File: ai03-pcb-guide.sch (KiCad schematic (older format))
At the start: 16 parts

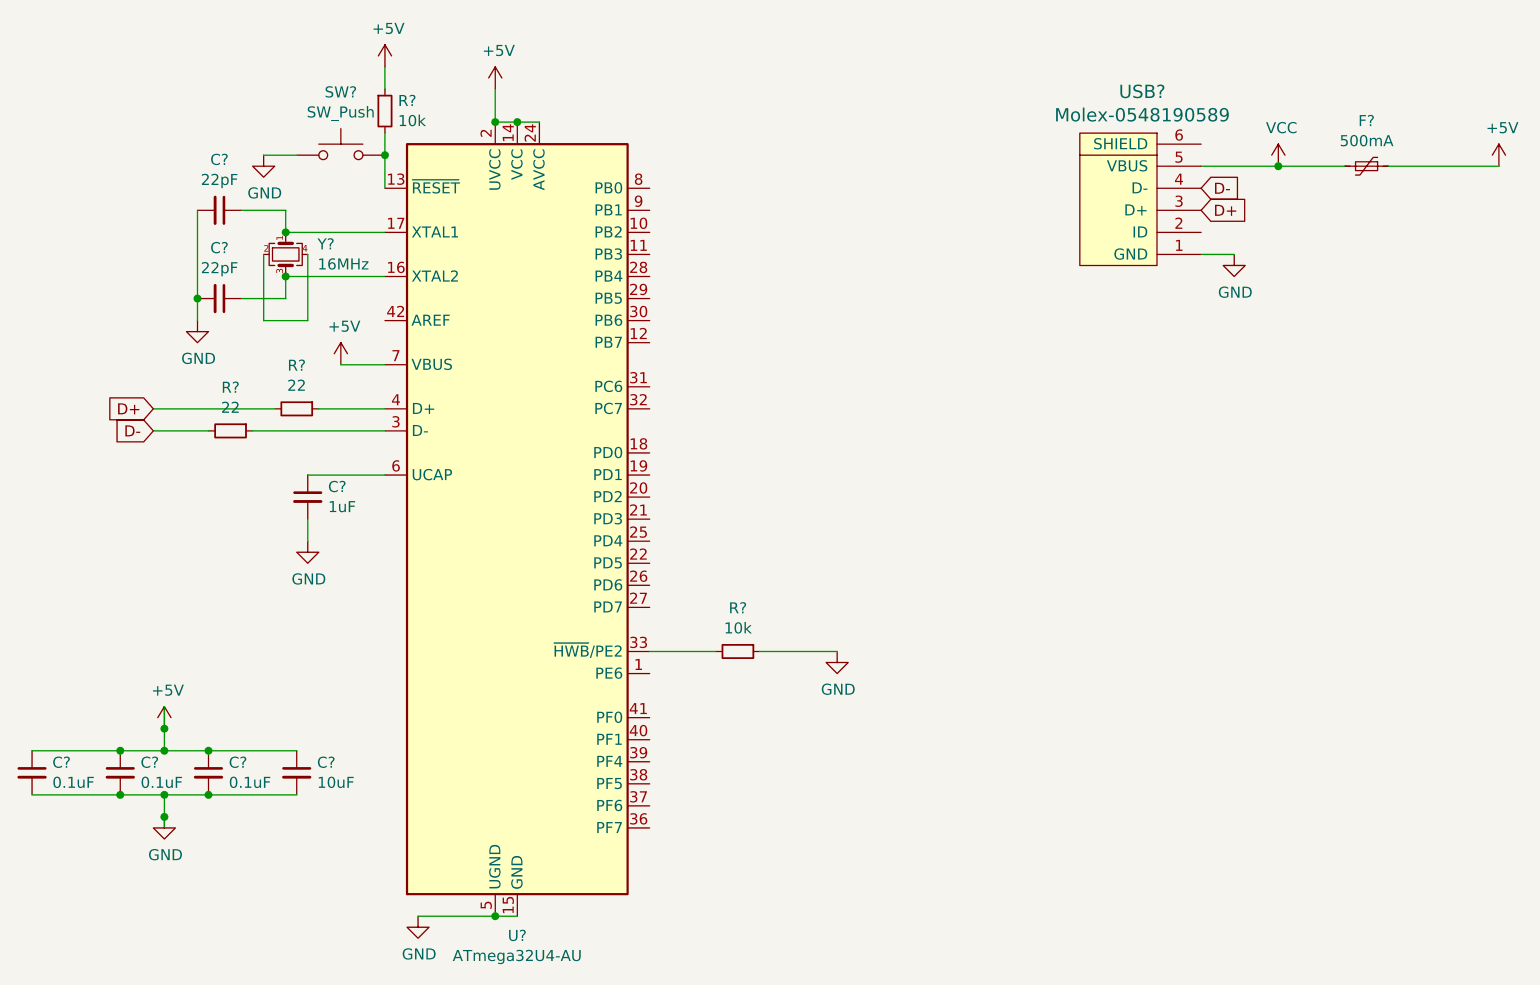
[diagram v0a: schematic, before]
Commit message: Switch schematic
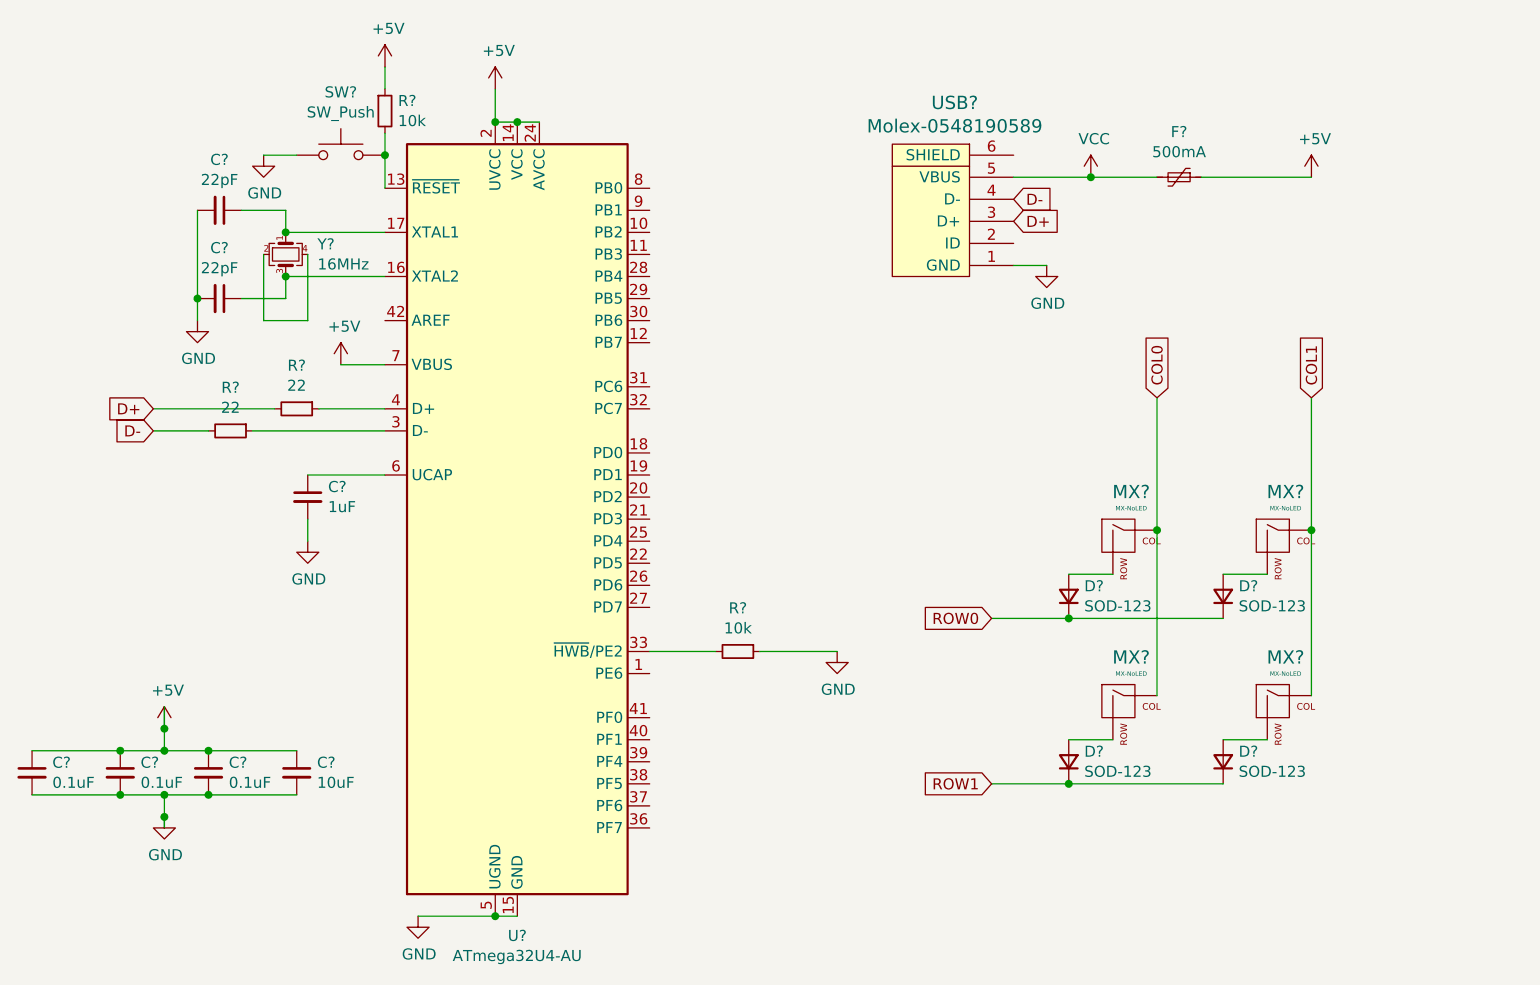
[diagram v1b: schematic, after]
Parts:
- added D? (x4): SOD-123, symbol Device:D_Small
- added MX? (x4): MX-NoLED, symbol MX_Alps_Hybrid:MX-NoLED
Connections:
- net labels added: COL0, COL1, ROW0, ROW1
- wire segments 45 -> 57
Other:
- moved on the sheet: F?, USB?
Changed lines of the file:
@@
 L random-keyboard-parts:Molex-0548190589 USB?
 U 1 1 6038615F
-P 6300 2400
-F 0 "USB?" V 6837 2367 60  0000 C CNN
-F 1 "Molex-0548190589" V 6731 2367 60  0000 C CNN
-F 2 "" H 6300 2400 60  0001 C CNN
-F 3 "" H 6300 2400 60  0001 C CNN
-	1    6300 2400
+P 5450 2450
+F 0 "USB?" V 5987 2417 60  0000 C CNN
+F 1 "Molex-0548190589" V 5881 2417 60  0000 C CNN
+F 2 "" H 5450 2450 60  0001 C CNN
+F 3 "" H 5450 2450 60  0001 C CNN
+	1    5450 2450
 	0    -1   -1   0
 $EndComp
@@
 L Device:Polyfuse_Small F?
 U 1 1 60388AFC
-P 7350 2200
-F 0 "F?" V 7145 2200 50  0000 C CNN
-F 1 "500mA" V 7236 2200 50  0000 C CNN
-F 2 "" H 7400 2000 50  0001 L CNN
-F 3 "~" H 7350 2200 50  0001 C CNN
-	1    7350 2200
+P 6500 2250
+F 0 "F?" V 6295 2250 50  0000 C CNN
+F 1 "500mA" V 6386 2250 50  0000 C CNN
+F 2 "" H 6550 2050 50  0001 L CNN
+F 3 "~" H 6500 2250 50  0001 C CNN
+	1    6500 2250
 	0    1    1    0
 $EndComp
 Wire Wire Line
-	6600 2200 6950 2200
+	5750 2250 6100 2250
 $Comp
 L power:VCC #PWR?
 U 1 1 6038C6B9
-P 6950 2200
-F 0 "#PWR?" H 6950 2050 50  0001 C CNN
-F 1 "VCC" H 6965 2373 50  0000 C CNN
-F 2 "" H 6950 2200 50  0001 C CNN
-F 3 "" H 6950 2200 50  0001 C CNN
-	1    6950 2200
+P 6100 2250
+F 0 "#PWR?" H 6100 2100 50  0001 C CNN
+F 1 "VCC" H 6115 2423 50  0000 C CNN
+F 2 "" H 6100 2250 50  0001 C CNN
+F 3 "" H 6100 2250 50  0001 C CNN
+	1    6100 2250
 	1    0    0    -1
 $EndComp
-Connection ~ 6950 2200
+Connection ~ 6100 2250
 Wire Wire Line
-	6950 2200 7250 2200
+	6100 2250 6400 2250
 Wire Wire Line
-	7450 2200 7950 2200
+	6600 2250 7100 2250
 $Comp
 L power:+5V #PWR?
 U 1 1 6038A873
-P 7950 2200
-F 0 "#PWR?" H 7950 2050 50  0001 C CNN
-F 1 "+5V" H 7965 2373 50  0000 C CNN
-F 2 "" H 7950 2200 50  0001 C CNN
-F 3 "" H 7950 2200 50  0001 C CNN
-	1    7950 2200
+P 7100 2250
+F 0 "#PWR?" H 7100 2100 50  0001 C CNN
+F 1 "+5V" H 7115 2423 50  0000 C CNN
+F 2 "" H 7100 2250 50  0001 C CNN
+F 3 "" H 7100 2250 50  0001 C CNN
+	1    7100 2250
 	1    0    0    -1
 $EndComp
-Text GLabel 6600 2400 2    50   Input ~ 0
+Text GLabel 5750 2450 2    50   Input ~ 0
 D+
-Text GLabel 6600 2300 2    50   Input ~ 0
+Text GLabel 5750 2350 2    50   Input ~ 0
 D-
 $Comp
 L power:GND #PWR?
 U 1 1 60394008
-P 6750 2600
-F 0 "#PWR?" H 6750 2350 50  0001 C CNN
-F 1 "GND" H 6755 2427 50  0000 C CNN
-F 2 "" H 6750 2600 50  0001 C CNN
-F 3 "" H 6750 2600 50  0001 C CNN
-	1    6750 2600
+P 5900 2650
+F 0 "#PWR?" H 5900 2400 50  0001 C CNN
+F 1 "GND" H 5905 2477 50  0000 C CNN
+F 2 "" H 5900 2650 50  0001 C CNN
+F 3 "" H 5900 2650 50  0001 C CNN
+	1    5900 2650
 	1    0    0    -1
 $EndComp
 Wire Wire Line
-	6600 2600 6750 2600
+	5750 2650 5900 2650
+$Comp
+L MX_Alps_Hybrid:MX-NoLED MX?
+U 1 1 60395692
+P 6250 3900
+F 0 "MX?" H 6283 4123 60  0000 C CNN
+F 1 "MX-NoLED" H 6283 4049 20  0000 C CNN
+F 2 "" H 5625 3875 60  0001 C CNN
+F 3 "" H 5625 3875 60  0001 C CNN
+	1    6250 3900
+	1    0    0    -1
+$EndComp
+$Comp
+L Device:D_Small D?
+U 1 1 6039B382
+P 6000 4150
+F 0 "D?" V 6046 4080 50  0000 R CNN
+F 1 "SOD-123" V 5955 4080 50  0000 R CNN
+F 2 "" V 6000 4150 50  0001 C CNN
+F 3 "~" V 6000 4150 50  0001 C CNN
+	1    6000 4150
+	0    -1   -1   0
+$EndComp
+Wire Wire Line
+	6200 4050 6000 4050
+$Comp
+L MX_Alps_Hybrid:MX-NoLED MX?
+U 1 1 603A0BDE
+P 6950 3900
+F 0 "MX?" H 6983 4123 60  0000 C CNN
+F 1 "MX-NoLED" H 6983 4049 20  0000 C CNN
+F 2 "" H 6325 3875 60  0001 C CNN
+F 3 "" H 6325 3875 60  0001 C CNN
+	1    6950 3900
+	1    0    0    -1
+$EndComp
+$Comp
+L Device:D_Small D?
+U 1 1 603A17C0
+P 6700 4150
+F 0 "D?" V 6746 4080 50  0000 R CNN
+F 1 "SOD-123" V 6655 4080 50  0000 R CNN
+F 2 "" V 6700 4150 50  0001 C CNN
+F 3 "~" V 6700 4150 50  0001 C CNN
+	1    6700 4150
+	0    -1   -1   0
+$EndComp
+Wire Wire Line
+	6900 4050 6700 4050
+$Comp
+L MX_Alps_Hybrid:MX-NoLED MX?
+U 1 1 603A2C50
+P 6250 4650
+F 0 "MX?" H 6283 4873 60  0000 C CNN
+F 1 "MX-NoLED" H 6283 4799 20  0000 C CNN
+F 2 "" H 5625 4625 60  0001 C CNN
+F 3 "" H 5625 4625 60  0001 C CNN
+	1    6250 4650
+	1    0    0    -1
+$EndComp
+$Comp
+L Device:D_Small D?
+U 1 1 603A36D6
+P 6000 4900
+F 0 "D?" V 6046 4830 50  0000 R CNN
+F 1 "SOD-123" V 5955 4830 50  0000 R CNN
+F 2 "" V 6000 4900 50  0001 C CNN
+F 3 "~" V 6000 4900 50  0001 C CNN
+	1    6000 4900
+	0    -1   -1   0
+$EndComp
+Wire Wire Line
+	6200 4800 6000 4800
+$Comp
+L MX_Alps_Hybrid:MX-NoLED MX?
+U 1 1 603A4940
+P 6950 4650
+F 0 "MX?" H 6983 4873 60  0000 C CNN
+F 1 "MX-NoLED" H 6983 4799 20  0000 C CNN
+F 2 "" H 6325 4625 60  0001 C CNN
+F 3 "" H 6325 4625 60  0001 C CNN
+	1    6950 4650
+	1    0    0    -1
+$EndComp
+$Comp
+L Device:D_Small D?
+U 1 1 603A51B7
+P 6700 4900
+F 0 "D?" V 6746 4830 50  0000 R CNN
+F 1 "SOD-123" V 6655 4830 50  0000 R CNN
+F 2 "" V 6700 4900 50  0001 C CNN
+F 3 "~" V 6700 4900 50  0001 C CNN
+	1    6700 4900
+	0    -1   -1   0
+$EndComp
+Wire Wire Line
+	6900 4800 6700 4800
+Wire Wire Line
+	7100 4600 7100 3850
+Connection ~ 7100 3850
+Wire Wire Line
+	7100 3850 7100 3250
+Wire Wire Line
+	6400 4600 6400 3850
+Connection ~ 6400 3850
+Wire Wire Line
+	6400 3850 6400 3250
+Wire Wire Line
+	6700 4250 6000 4250
+Connection ~ 6000 4250
+Wire Wire Line
+	6000 4250 5650 4250
+Wire Wire Line
+	6700 5000 6000 5000
+Connection ~ 6000 5000
+Wire Wire Line
+	6000 5000 5650 5000
+Text GLabel 6400 3250 1    50   Input ~ 0
+COL0
+Text GLabel 7100 3250 1    50   Input ~ 0
+COL1
+Text GLabel 5650 4250 0    50   Input ~ 0
+ROW0
+Text GLabel 5650 5000 0    50   Input ~ 0
+ROW1
 $EndSCHEMATC
